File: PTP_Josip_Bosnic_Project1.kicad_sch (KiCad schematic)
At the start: 25 parts, among them J1 Screw_Terminal_01x02, SW1 SW_Push, SW2 SW_SPDT_312, U1 LM2574N-5, U6 74LVC1G11, U7 NE555P

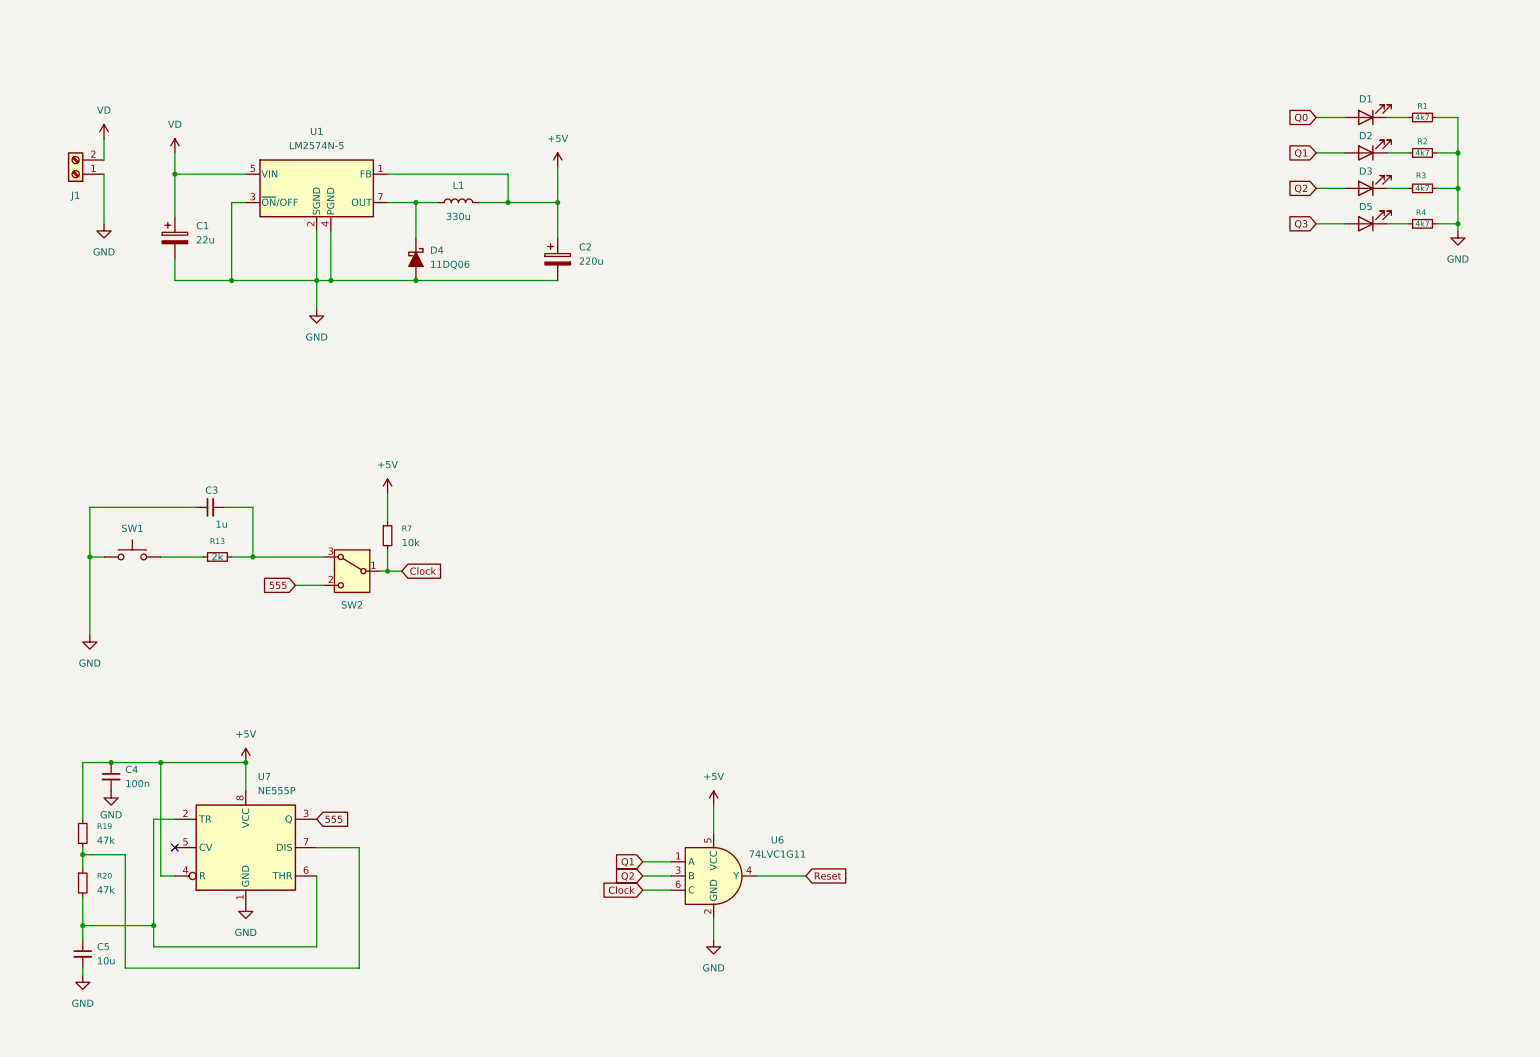
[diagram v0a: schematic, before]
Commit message: LV4
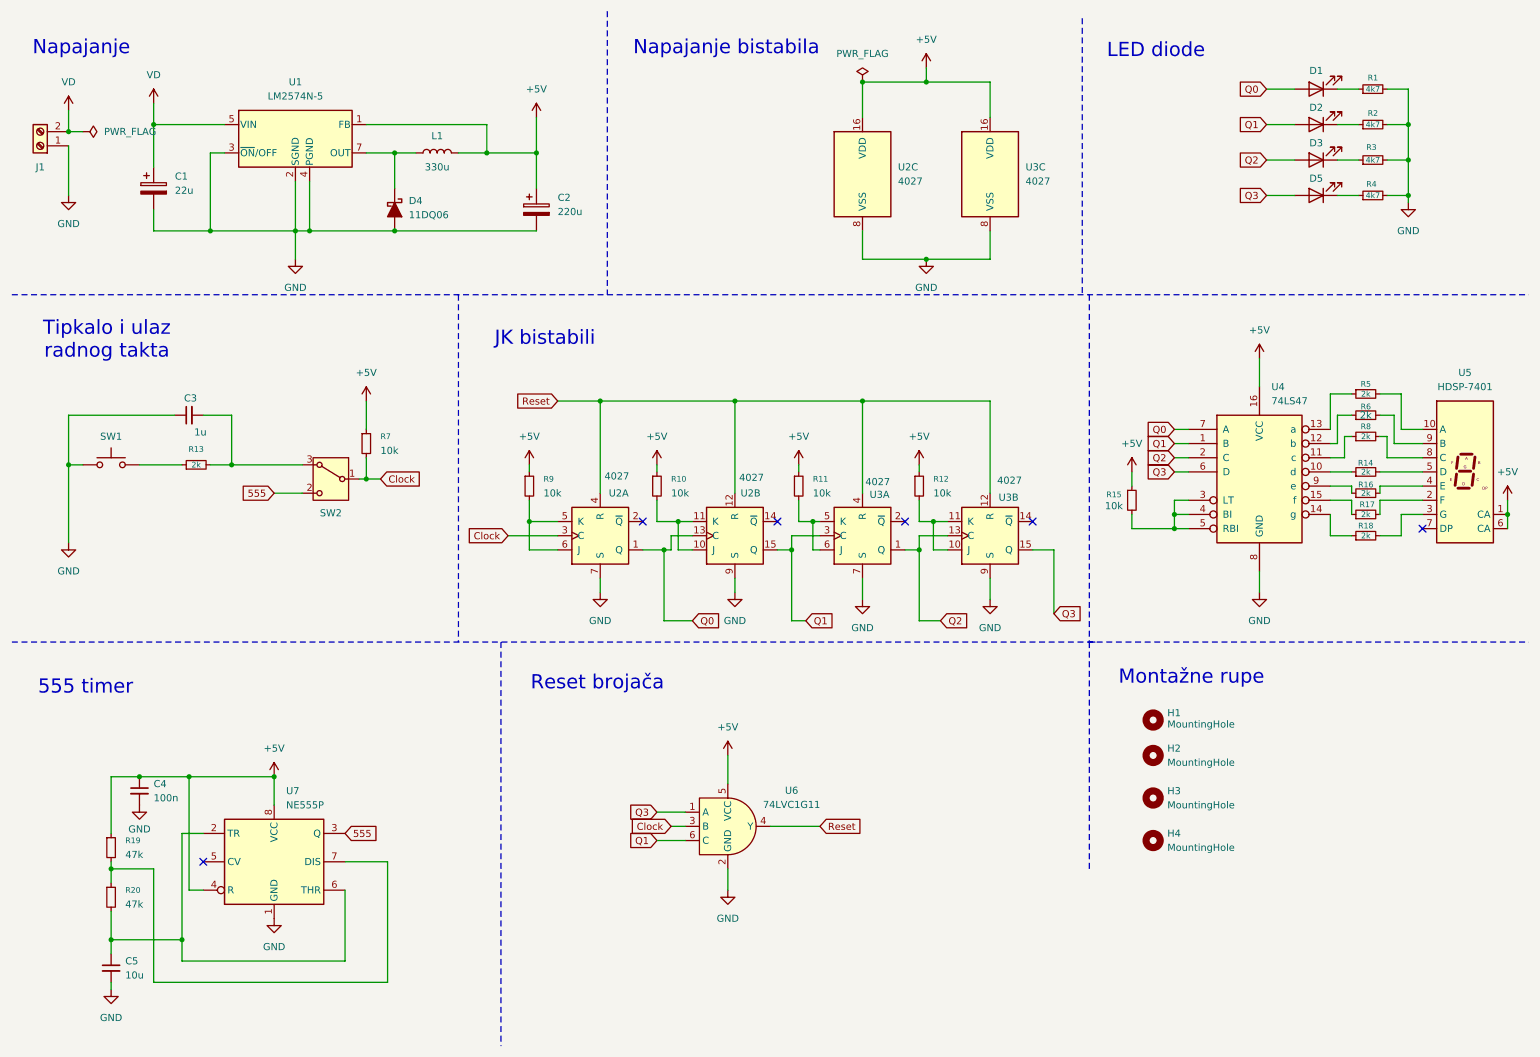
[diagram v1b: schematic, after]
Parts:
- added H1, H2, H3, H4: MountingHole, symbol Mechanical:MountingHole
- added R10, R11, R12, R9: 10k, Resistor_SMD:R_1206_3216Metric_Pad1.30x1.75mm_HandSolder, symbol Device:R_Small
- added R14, R16, R17, R18, R5, R6, R8: 2k, symbol Device:R_Small
- added R15: 10k, symbol Device:R_Small
- added U2: 4027, Package_DIP:DIP-16_W7.62mm_Socket_LongPads, symbol 4xxx:4027
- added U3: 4027, symbol 4xxx:4027
- added U4: 74LS47, symbol 74xx:74LS47
- added U5: HDSP-7401, Display_7Segment:HDSP-7401, symbol Display_Character:HDSP-7401
- C1: footprint (none) -> Capacitor_THT:CP_Radial_D5.0mm_P2.00mm; Manufacturer  (none) -> AISHI; Manufacturer Part Number  (none) -> EWH1EM220D11OT
- C3: footprint (none) -> Capacitor_SMD:C_1206_3216Metric_Pad1.33x1.80mm_HandSolder; Manufacturer  (none) -> SAMSUNG; Manufacturer Part Number  (none) -> CL31B105KBHNNNE
- C4: footprint (none) -> Capacitor_SMD:C_1206_3216Metric_Pad1.33x1.80mm_HandSolder; Manufacturer  (none) -> SAMSUNG; Manufacturer Part Number  (none) -> CL31B104KBCNNNC
- C5: footprint (none) -> Capacitor_SMD:C_1206_3216Metric_Pad1.33x1.80mm_HandSolder; Manufacturer (none) -> SAMSUNG; Manufacturer Part Number (none) -> CL31A106KBHNNNE
- J1: footprint (none) -> TerminalBlock_MetzConnect:TerminalBlock_MetzConnect_Type011_RT05502HBLC_1x02_P5.00mm_Horizontal; Manufacturer  (none) -> DEGSON ELECTRONICS; Manufacturer Part Number  (none) -> DG301-5.0-02P-12-00A(H)
- R13: footprint (none) -> Resistor_SMD:R_1206_3216Metric_Pad1.30x1.75mm_HandSolder; Manufacturer (none) -> ROYALOHM; Manufacturer Part Number  (none) -> 1206S4F2001T5E
- R19: footprint (none) -> Resistor_SMD:R_1206_3216Metric_Pad1.30x1.75mm_HandSolder; Manufacturer  (none) -> ROYALOHM; Manufacturer Part Number  (none) -> 1206S4J0473T5E
- R20: footprint (none) -> Resistor_SMD:R_1206_3216Metric_Pad1.30x1.75mm_HandSolder; Manufacturer (none) -> ROYALOHM; Manufacturer Part Number (none) -> 1206S4J0473T5E
- R7: footprint (none) -> Resistor_SMD:R_1206_3216Metric_Pad1.30x1.75mm_HandSolder
- SW1: footprint (none) -> Button_Switch_THT:SW_PUSH_6mm_H4.3mm; Manufacturer  (none) -> microswitch TACT; Manufacturer Part Number  (none) -> TACT-64N-F
- U1: footprint Package_DIP:DIP-8_W7.62mm -> Package_DIP:DIP-8_W7.62mm_Socket_LongPads; Manufacturer  (none) -> ONSEMI
- U6: Manufacturer (none) -> TEXAS INSTRUMENTS; Manufacturer Part Number  (none) -> SN74LVC1G11DBVR
- U7: Manufacturer  (none) -> TEXAS INSTRUMENTS; Manufacturer Part Number  (none) -> NE555P
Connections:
- net +5V: now also R10.1, R11.1, R12.1, R15.1, R9.1, U2.16 (VDD), U3.16 (VDD), U4.16 (VCC), U5.1 (CA), U5.6 (CA)
- net Clock: now also U6.3 (B), U2.3 (C); no longer U6.6 (C)
- net GND: now also U2.7 (S), U2.8 (VSS), U2.9 (S), U3.7 (S), U3.8 (VSS), U3.9 (S), U4.8 (GND)
- net Q0: now also U2.1 (Q), U2.13 (C), U4.7 (A)
- net Q1: now also U6.6 (C), U2.15 (Q), U3.3 (C), U4.1 (B); no longer U6.1 (A)
- net Q2: now also U3.1 (Q), U3.13 (C), U4.2 (C); no longer U6.3 (B)
- net Q3: now also U6.1 (A), U3.15 (Q), U4.6 (D)
- net Reset: now also U2.12 (R), U2.4 (R), U3.12 (R), U3.4 (R)
- new net: R11.2, U3.5 (K), U3.6 (J)
- new net: R12.2, U3.10 (J), U3.11 (K)
- new net: R10.2, U2.10 (J), U2.11 (K)
- new net: R5.1, U4.13 (a)
- new net: R5.2, U5.10 (A)
- new net: R14.1, U4.10 (d)
- new net: R14.2, U5.5 (D)
- new net: R17.1, U4.15 (f)
- new net: R17.2, U5.2 (F)
- new net: R8.1, U4.11 (c)
- new net: R6.1, U4.12 (b)
- new net: R18.1, U4.14 (g)
- new net: R15.2, U4.3 (LT), U4.4 (BI), U4.5 (RBI)
- new net: R16.1, U4.9 (e)
- new net: R6.2, U5.9 (B)
- new net: R16.2, U5.4 (E)
- new net: R18.2, U5.3 (G)
- new net: R8.2, U5.8 (C)
- new net: R9.2, U2.5 (K), U2.6 (J)
- no-connect marks 1 -> 6
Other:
- note added: "555 timer"
- note added: "JK bistabili"
- note added: "LED diode"
- note added: "Montažne rupe"
- note added: "Napajanje"
- note added: "Napajanje bistabila"
- note added: "Reset brojača"
- note added: "Tipkalo i ulaz radnog takta"
- moved on the sheet: C1, C2, C3, C4, C5, D1, D2, D3, D4, D5, J1, L1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

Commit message: Zadaca
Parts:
- C2: footprint (none) -> Capacitor_THT:CP_Radial_D5.0mm_P2.00mm; Manufacturer  (none) -> SAMWHA; Manufacturer Part Number  (none) -> RD1A227M05011BB
- D1, D2, D3, D5: footprint (none) -> LED_THT:LED_D5.0mm
- D4: footprint (none) -> Diode_THT:D_DO-41_SOD81_P12.70mm_Horizontal; Manufacturer  (none) -> SMC DIODE SOLUTIONS; Manufacturer Part Number  (none) -> 11DQ06TA
- H1, H2, H3, H4: footprint (none) -> MountingHole:MountingHole_5.5mm
- L1: footprint (none) -> Inductor_THT:L_Radial_D7.2mm_P3.00mm_Murata_1700; Manufacturer  (none) -> FERROCORE; Manufacturer Part Number  (none) -> COIL0608-0.33
- R1, R2, R3, R4: footprint (none) -> Resistor_THT:R_Axial_DIN0207_L6.3mm_D2.5mm_P10.16mm_Horizontal
- R14, R16, R17, R18, R5, R6, R8: footprint (none) -> Resistor_SMD:R_1206_3216Metric_Pad1.30x1.75mm_HandSolder; Manufacturer  (none) -> ROYALOHM; Manufacturer Part Number  (none) -> 1206S4F2001T5E
- R15: footprint (none) -> Resistor_SMD:R_1206_3216Metric_Pad1.30x1.75mm_HandSolder
- SW2: footprint (none) -> Button_Switch_THT:SW_Slide_SPDT_Straight_CK_OS102011MS2Q; Manufacturer  (none) -> C&K; Manufacturer Part Number  (none) -> OS102011MS2QN1C
- U1: Manufacturer Part Number  (none) -> LM2574N-5G
- U3: footprint (none) -> Package_DIP:DIP-16_W7.62mm_Socket_LongPads; Manufacturer  (none) -> RENESAS; Manufacturer Part Number  (none) -> CD4027BMS
- U4: footprint (none) -> Package_DIP:DIP-16_W7.62mm_Socket_LongPads; Manufacturer  (none) -> TEXAS INSTRUMENTS; Manufacturer Part Number  (none) -> SN74LS47N
- U5: Manufacturer  (none) -> FORYARD; Manufacturer Part Number (none) -> FYS-3911BUHR-21
- U6: footprint SOT-23-6:SOT-23-6 -> Package_TO_SOT_SMD:SOT-23-6
